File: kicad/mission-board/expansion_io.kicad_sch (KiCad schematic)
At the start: 5 parts, among them J14 I2C Expansion, J15 SPI Expansion, J16 GPIO/ADC Expansion, J17 Debug UART, J18 Inter-ESP UART

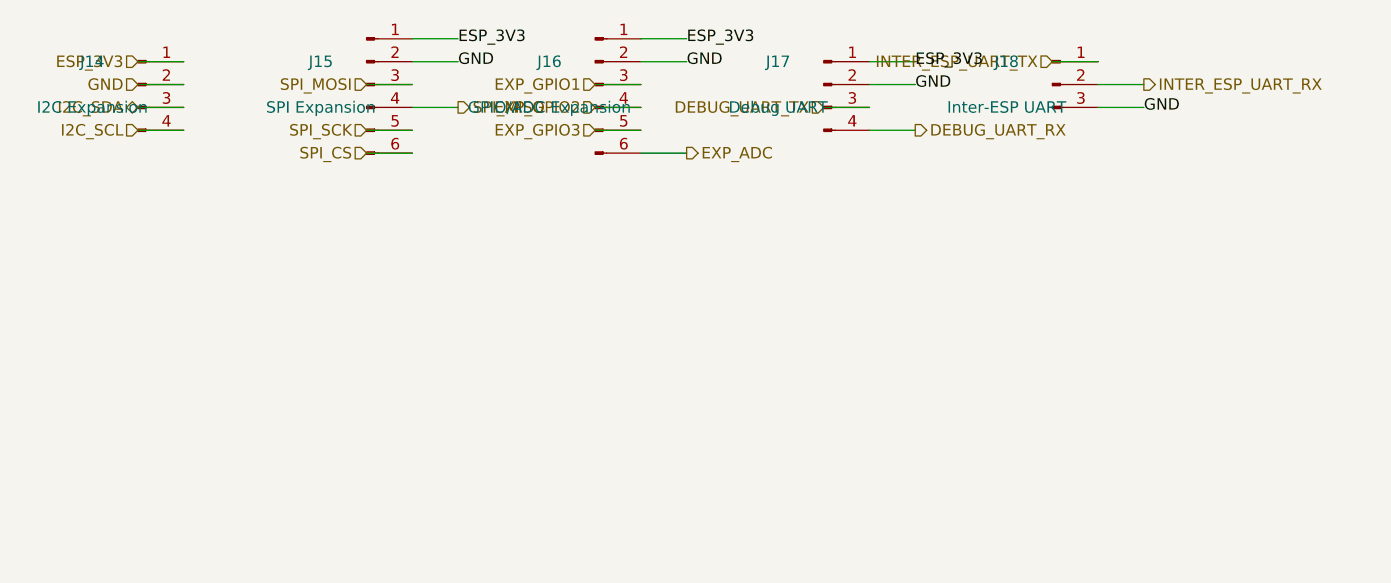
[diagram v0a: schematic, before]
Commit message: pcb progress
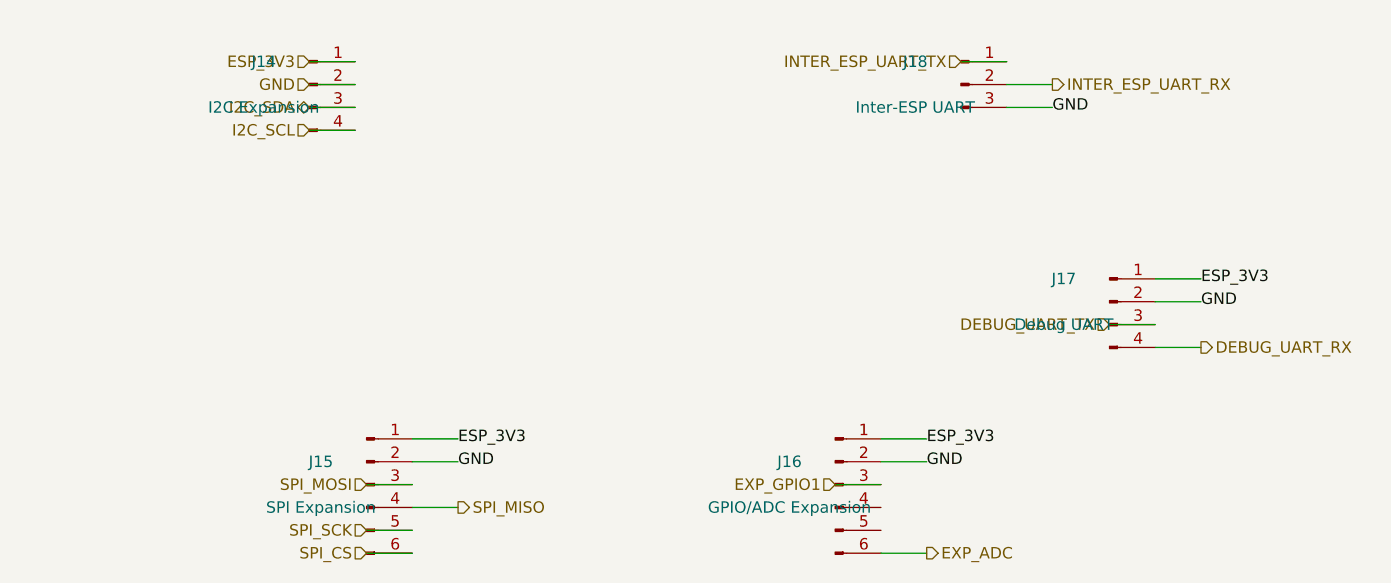
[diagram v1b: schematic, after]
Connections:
- net EXP_GPIO2: no longer names the net of J16.4 (Pin_4)
- net EXP_GPIO3: no longer names the net of J16.5 (Pin_5)
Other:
- moved on the sheet: J14, J15, J16, J17, J18

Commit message: progress on v1 of mission board
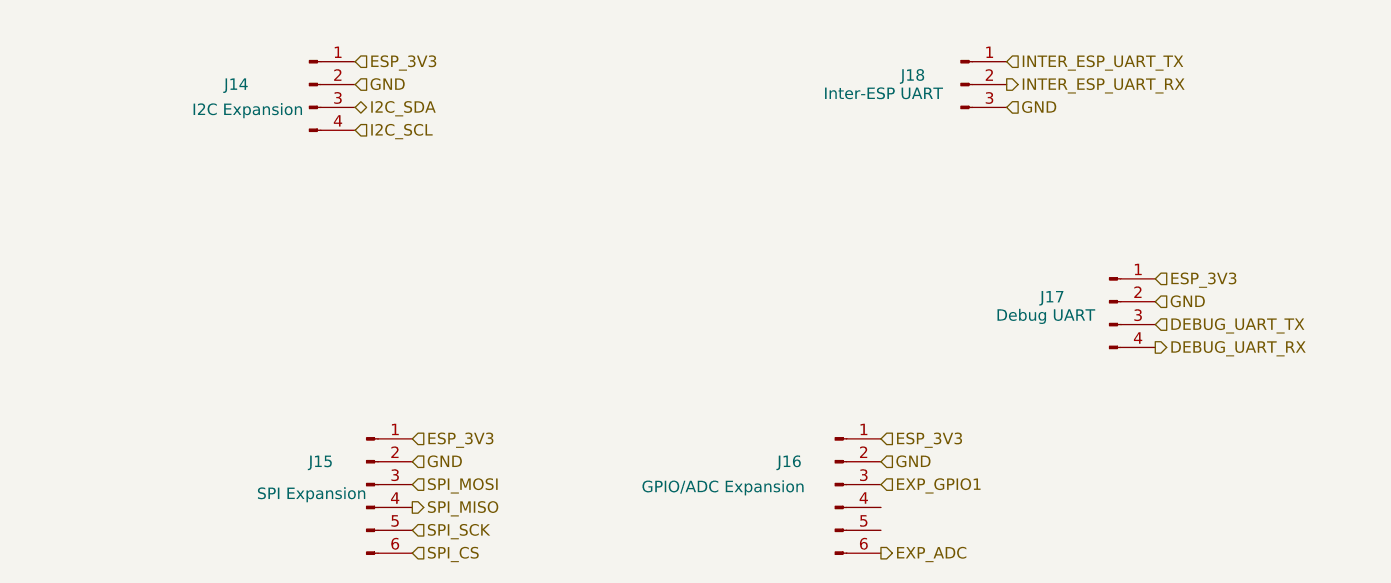
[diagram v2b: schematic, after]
